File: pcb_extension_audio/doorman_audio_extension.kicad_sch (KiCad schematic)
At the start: 38 parts, among them J1 Audio Out, J2 GPIO, J4 Extension Board Connector, J5 Audio In, U1 ES8388

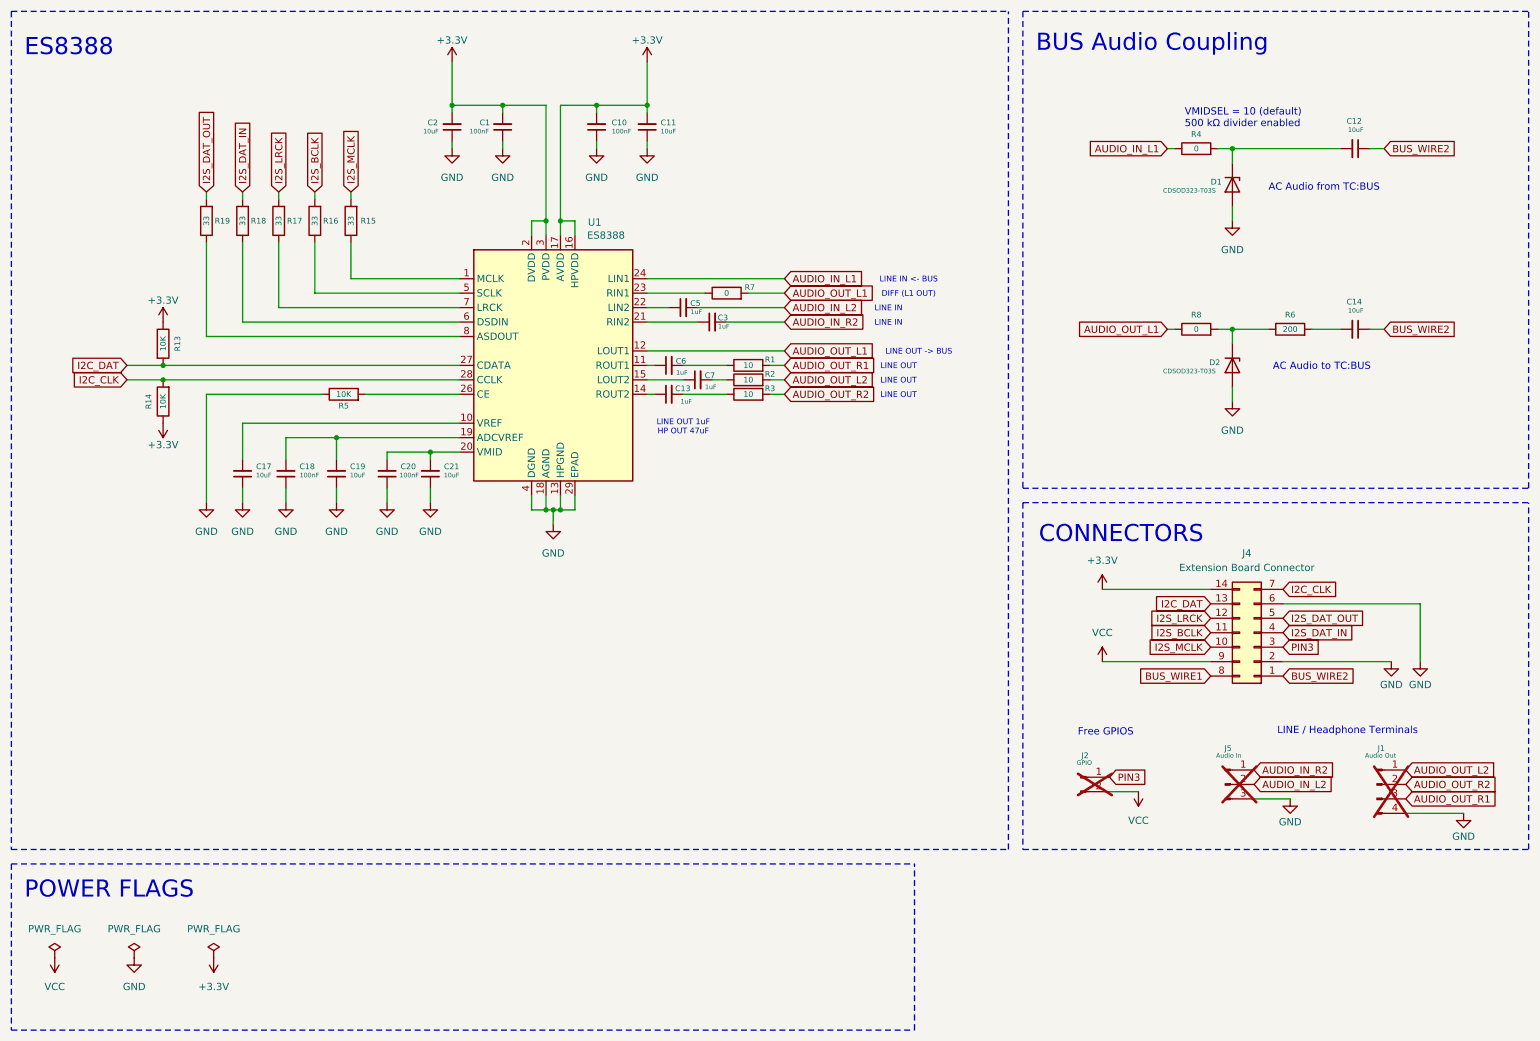
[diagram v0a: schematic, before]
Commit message: WIP
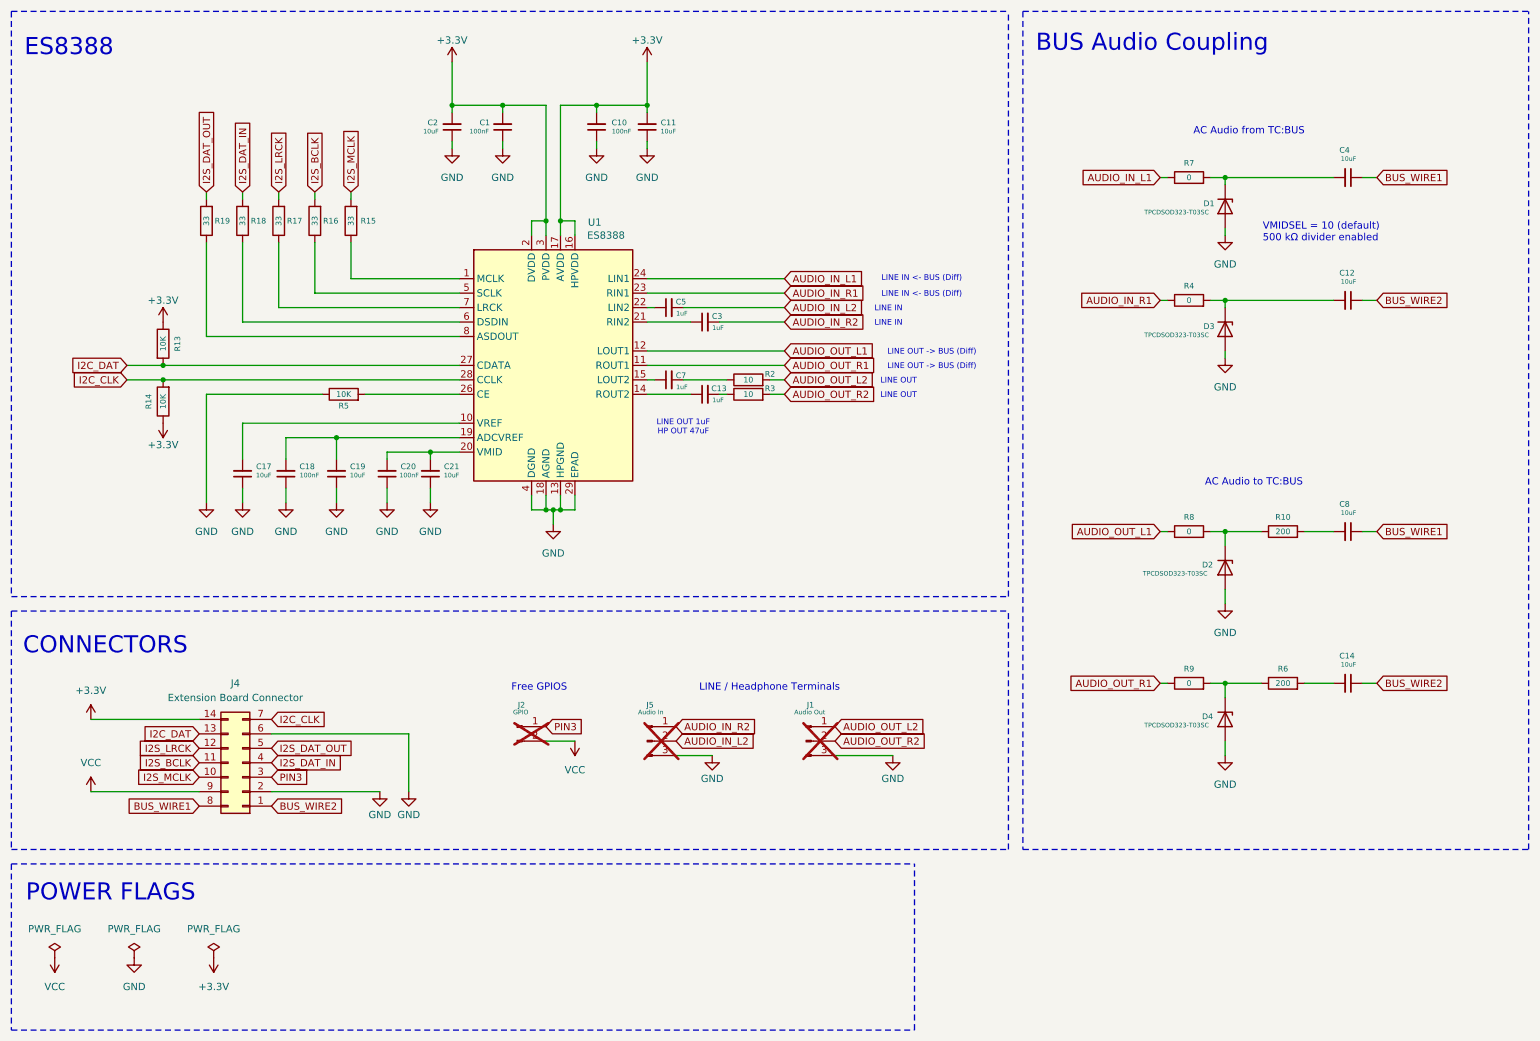
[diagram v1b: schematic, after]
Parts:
- removed C6: 1uF, Capacitor_SMD:C_0603_1608Metric, symbol Device:C_Small
- removed R1: 10, Resistor_SMD:R_0603_1608Metric, symbol Device:R
- added C4, C8: 10uF, Capacitor_SMD:C_1206_3216Metric, symbol Device:C_Small
- added D3, D4: TPCDSOD323-T03SC, Diode_SMD:D_SOD-323, symbol Diode:PTVS5V0Z1USK
- added R10: 200, Resistor_SMD:R_1206_3216Metric, symbol Device:R
- added R9: 0, Resistor_SMD:R_0603_1608Metric, symbol Device:R
- D1, D2: value CDSOD323-T03S -> TPCDSOD323-T03SC
- J1: footprint Connector_PinHeader_2.54mm:PinHeader_1x04_P2.54mm_Vertical -> Connector_PinHeader_2.54mm:PinHeader_1x03_P2.54mm_Vertical; symbol Connector:Conn_01x04_Pin -> Connector:Conn_01x03_Pin; now in the parts list
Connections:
- net AUDIO_IN_L1: now also R7.1; no longer R4.1
- net AUDIO_OUT_L1: no longer R7.2
- net AUDIO_OUT_R1: now also U1.11 (ROUT1), R9.1; no longer J1.3 (Pin_3)
- net BUS_WIRE1: now also C4.1, C8.1
- net GND: now also J1.3 (Pin_3), D3.2 (A), D4.2 (A); no longer J1.4 (Pin_4)
- net at D2.1 (K), R8.2: now also R10.1; no longer R6.1
- net AUDIO_IN_R1: now reaches U1.23 (RIN1)
- net AUDIO_IN_R1: now also R4.1; no longer R7.1
- net at C12.2, R4.2: now also D3.1 (K); no longer D1.1 (K)
- new net: C4.2, D1.1 (K), R7.2
- new net: D4.1 (K), R6.1, R9.2
- new net: C8.2, R10.2
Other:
- note added: "LINE IN <- BUS (Diff)"
- note added: "LINE OUT -> BUS (Diff)"
- note removed: "DIFF (L1 OUT)"
- note removed: "LINE IN <- BUS"
- note removed: "LINE OUT -> BUS"
- moved on the sheet: C12, C13, C14, C3, C5, C7, D1, D2, J2, J4, J5, R6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
